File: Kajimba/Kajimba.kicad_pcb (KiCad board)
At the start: 2 copper layers, 86.4 x 49.5 mm, 17 parts, among them J1 Barrel_Jack, J2 Flow sensor JST, J3 Screen, J4 Pump GND, J5 Button, J6 Conn_01x02_Female, K1 SANYOU_SRD_Form_C, Q1 BC547, SW1 Button, U1 Pico, U2 LM7805_TO220

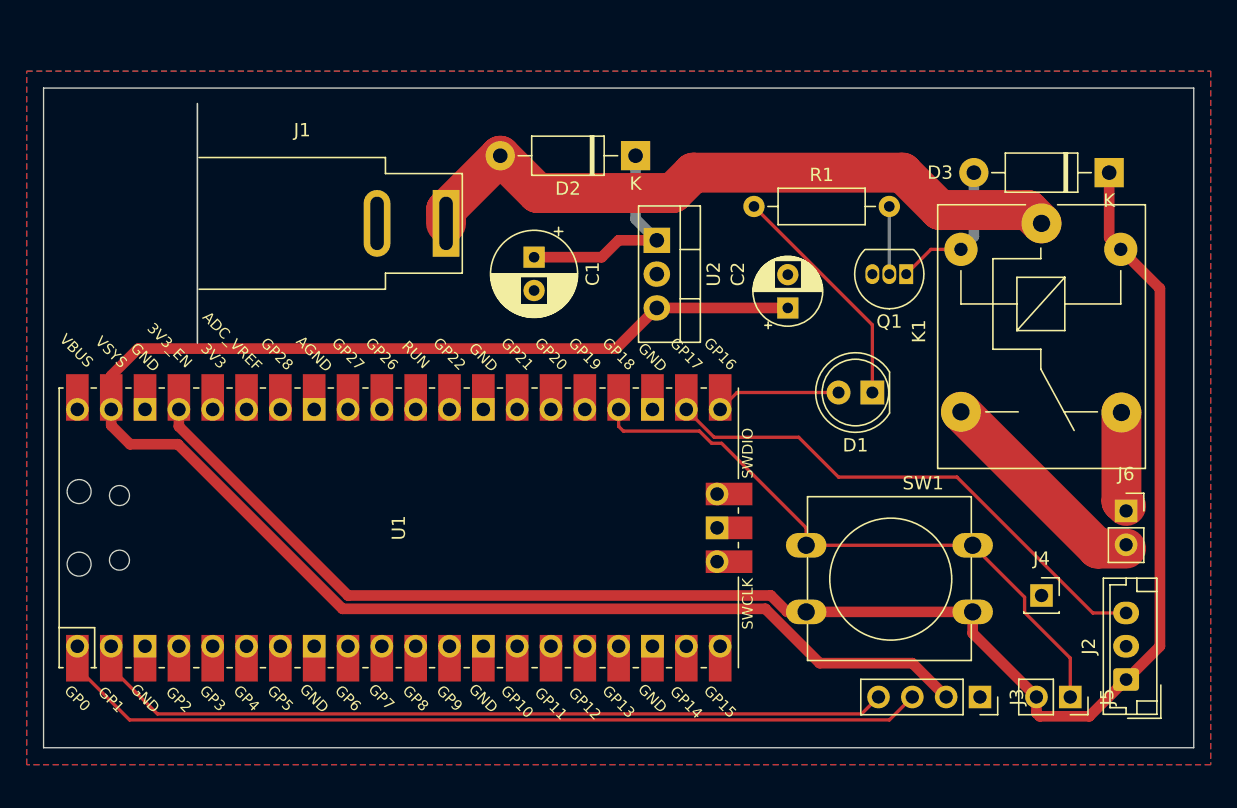
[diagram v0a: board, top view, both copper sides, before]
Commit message: KiCad PCB Pump v01.1
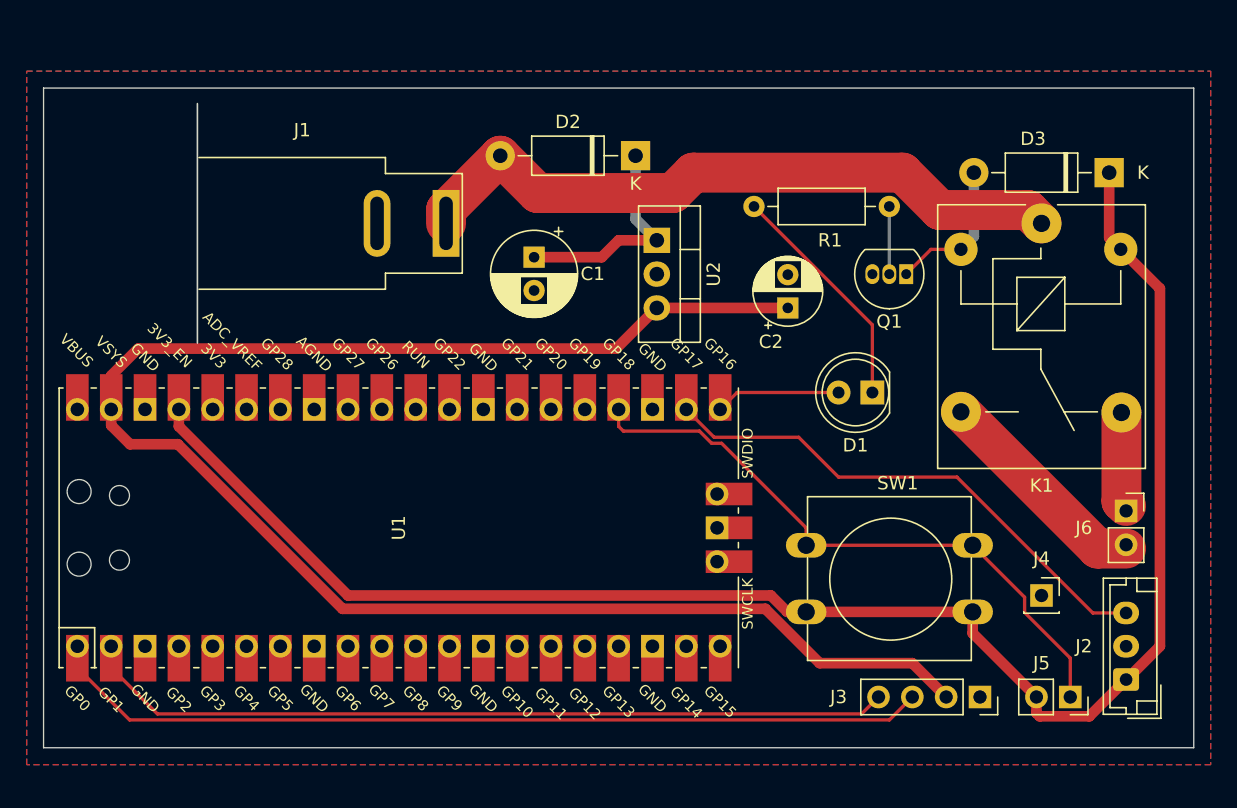
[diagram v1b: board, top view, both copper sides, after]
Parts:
- J2: value Flow sensor JST -> Flow sensor
- J6: value Conn_01x02_Female -> Relay out
- K1: value SANYOU_SRD_Form_C -> Relay
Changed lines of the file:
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@@
     (property "Sheetname" "")
     (attr through_hole)
-    (fp_text reference "D2" (at 5.08 -2.47) (layer "F.SilkS")
-      (effects (font (size 1 1) (thickness 0.15)))
-    )
-    (fp_text value "1N4007" (at 5.08 2.47) (layer "F.Fab")
+    (fp_text reference "D2" (at 5.08 2.54) (layer "F.SilkS")
+      (effects (font (size 1 1) (thickness 0.15)))
+    )
+    (fp_text value "1N4007" (at 5.08 -2.54) (layer "F.Fab")
       (effects (font (size 1 1) (thickness 0.15)))
     )
@@
     (property "Sheetname" "")
     (attr through_hole)
-    (fp_text reference "C1" (at 1.25 -4.4 90) (layer "F.SilkS")
-      (effects (font (size 1 1) (thickness 0.15)))
-    )
-    (fp_text value "470uF" (at 1.25 4.4 90) (layer "F.Fab")
+    (fp_text reference "C1" (at 1.25 -4.4 180) (layer "F.SilkS")
+      (effects (font (size 1 1) (thickness 0.15)))
+    )
+    (fp_text value "470uF" (at -3.175 0 180) (layer "F.Fab")
       (effects (font (size 1 1) (thickness 0.15)))
     )
@@
     (property "Sheetname" "")
     (attr through_hole)
-    (fp_text reference "J5" (at 0 -2.77 -90) (layer "F.SilkS")
-      (effects (font (size 1 1) (thickness 0.15)))
-    )
-    (fp_text value "Button" (at 0 5.31 -90) (layer "F.Fab")
+    (fp_text reference "J5" (at -2.54 2.159) (layer "F.SilkS")
+      (effects (font (size 1 1) (thickness 0.15)))
+    )
+    (fp_text value "Button" (at 2.54 1.524) (layer "F.Fab")
       (effects (font (size 1 1) (thickness 0.15)))
     )
@@
     (property "Sheetname" "")
     (attr through_hole)
-    (fp_text reference "J2" (at 2.5 -2.8 90) (layer "F.SilkS")
-      (effects (font (size 1 1) (thickness 0.15)))
-    )
-    (fp_text value "Flow sensor JST" (at 2.5 3.4 90) (layer "F.Fab")
+    (fp_text reference "J2" (at 2.5 -3.175 180) (layer "F.SilkS")
+      (effects (font (size 1 1) (thickness 0.15)))
+    )
+    (fp_text value "Flow sensor" (at 2.5 3.81 90) (layer "F.Fab")
       (effects (font (size 1 1) (thickness 0.15)))
     )
@@
     (property "Sheetname" "")
     (attr through_hole)
-    (fp_text reference "K1" (at 8.1 9.2 90) (layer "F.SilkS")
-      (effects (font (size 1 1) (thickness 0.15)))
-    )
-    (fp_text value "SANYOU_SRD_Form_C" (at 19.05 0 180) (layer "F.Fab")
+    (fp_text reference "K1" (at 19.685 0 180) (layer "F.SilkS")
+      (effects (font (size 1 1) (thickness 0.15)))
+    )
+    (fp_text value "Relay" (at 19.685 -1.27 180) (layer "F.Fab")
       (effects (font (size 1 1) (thickness 0.15)))
     )
@@
       (effects (font (size 1 1) (thickness 0.15)))
     )
-    (fp_text value "Barrel_Jack" (at -11 9.9) (layer "F.Fab")
+    (fp_text value "Barrel_Jack" (at -2.915 7.62) (layer "F.Fab")
       (effects (font (size 1 1) (thickness 0.15)))
     )
@@
     (property "Sheetname" "")
     (attr through_hole)
-    (fp_text reference "SW1" (at 8.78 -4.66) (layer "F.SilkS")
-      (effects (font (size 1 1) (thickness 0.15)))
-    )
-    (fp_text value "Button" (at 2.43 9.93) (layer "F.Fab")
+    (fp_text reference "SW1" (at 6.875 -4.66) (layer "F.SilkS")
+      (effects (font (size 1 1) (thickness 0.15)))
+    )
+    (fp_text value "Button" (at 2.43 -4.485) (layer "F.Fab")
       (effects (font (size 1 1) (thickness 0.15)))
     )
@@
     (property "Sheetname" "")
     (attr through_hole)
-    (fp_text reference "J3" (at 0 -2.77 -90) (layer "F.SilkS")
-      (effects (font (size 1 1) (thickness 0.15)))
-    )
-    (fp_text value "Screen" (at 0 10.39 -90) (layer "F.Fab")
+    (fp_text reference "J3" (at 0 10.62) (layer "F.SilkS")
+      (effects (font (size 1 1) (thickness 0.15)))
+    )
+    (fp_text value "Screen" (at 2.54 3.635) (layer "F.Fab")
       (effects (font (size 1 1) (thickness 0.15)))
     )
@@
     (property "Sheetname" "")
     (attr through_hole)
-    (fp_text reference "J6" (at 0 -2.77) (layer "F.SilkS")
-      (effects (font (size 1 1) (thickness 0.15)))
-    )
-    (fp_text value "Conn_01x02_Female" (at 0 5.31) (layer "F.Fab")
+    (fp_text reference "J6" (at -3.175 1.27) (layer "F.SilkS")
+      (effects (font (size 1 1) (thickness 0.15)))
+    )
+    (fp_text value "Relay out" (at 3.81 0.635 90) (layer "F.Fab")
       (effects (font (size 1 1) (thickness 0.15)))
     )
@@
     (property "Sheetname" "")
     (attr through_hole)
-    (fp_text reference "R1" (at 5.08 -2.37) (layer "F.SilkS")
-      (effects (font (size 1 1) (thickness 0.15)))
-    )
-    (fp_text value "1.5k" (at 5.08 2.37) (layer "F.Fab")
+    (fp_text reference "R1" (at 5.715 2.54) (layer "F.SilkS")
+      (effects (font (size 1 1) (thickness 0.15)))
+    )
+    (fp_text value "1.5k" (at 5.08 -2.54) (layer "F.Fab")
       (effects (font (size 1 1) (thickness 0.15)))
     )
@@
     (property "Sheetname" "")
     (attr through_hole)
-    (fp_text reference "D3" (at 12.7 0) (layer "F.SilkS")
-      (effects (font (size 1 1) (thickness 0.15)))
-    )
-    (fp_text value "1N4007" (at 5.08 2.47) (layer "F.Fab")
-      (effects (font (size 1 1) (thickness 0.15)))
-    )
-    (fp_text user "K" (at 0 -2.1) (layer "F.SilkS")
+    (fp_text reference "D3" (at 5.715 2.54) (layer "F.SilkS")
+      (effects (font (size 1 1) (thickness 0.15)))
+    )
+    (fp_text value "1N4007" (at 1.905 2.54) (layer "F.Fab")
+      (effects (font (size 1 1) (thickness 0.15)))
+    )
+    (fp_text user "K" (at -2.54 0) (layer "F.SilkS")
       (effects (font (size 1 1) (thickness 0.15)))
     )
@@
     (property "Sheetname" "")
     (attr through_hole)
-    (fp_text reference "C2" (at 2.54 -3.75 90) (layer "F.SilkS")
-      (effects (font (size 1 1) (thickness 0.15)))
-    )
-    (fp_text value "1uF" (at 1.25 3.75 90) (layer "F.Fab")
+    (fp_text reference "C2" (at -2.54 -1.27 180) (layer "F.SilkS")
+      (effects (font (size 1 1) (thickness 0.15)))
+    )
+    (fp_text value "1uF" (at -2.54 1.27 180) (layer "F.Fab")
       (effects (font (size 1 1) (thickness 0.15)))
     )
@@
     (connect_pads (clearance 0))
     (min_thickness 0.254)
-    (keepout (tracks not_allowed) (vias not_allowed) (pads not_allowed) (copperpour not_allowed) (footprints allowed))
+    (keepout (tracks not_allowed) (vias not_allowed) (pads not_allowed ) (copperpour not_allowed) (footprints allowed))
     (fill (thermal_gap 0.508) (thermal_bridge_width 0.508))
     (polygon
@@
     (connect_pads (clearance 0))
     (min_thickness 0.254)
-    (keepout (tracks not_allowed) (vias allowed) (pads allowed) (copperpour not_allowed) (footprints allowed))
+    (keepout (tracks not_allowed) (vias allowed) (pads allowed ) (copperpour not_allowed) (footprints allowed))
     (fill (thermal_gap 0.508) (thermal_bridge_width 0.508))
     (polygon
@@
     (connect_pads (clearance 0))
     (min_thickness 0.254)
-    (keepout (tracks not_allowed) (vias not_allowed) (pads not_allowed) (copperpour not_allowed) (footprints allowed))
+    (keepout (tracks not_allowed) (vias not_allowed) (pads not_allowed ) (copperpour not_allowed) (footprints allowed))
     (fill (thermal_gap 0.508) (thermal_bridge_width 0.508))
     (polygon
@@
     (connect_pads (clearance 0))
     (min_thickness 0.254)
-    (keepout (tracks not_allowed) (vias not_allowed) (pads not_allowed) (copperpour not_allowed) (footprints allowed))
+    (keepout (tracks not_allowed) (vias not_allowed) (pads not_allowed ) (copperpour not_allowed) (footprints allowed))
     (fill (thermal_gap 0.508) (thermal_bridge_width 0.508))
     (polygon

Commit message: KiCad PCB Pump v02
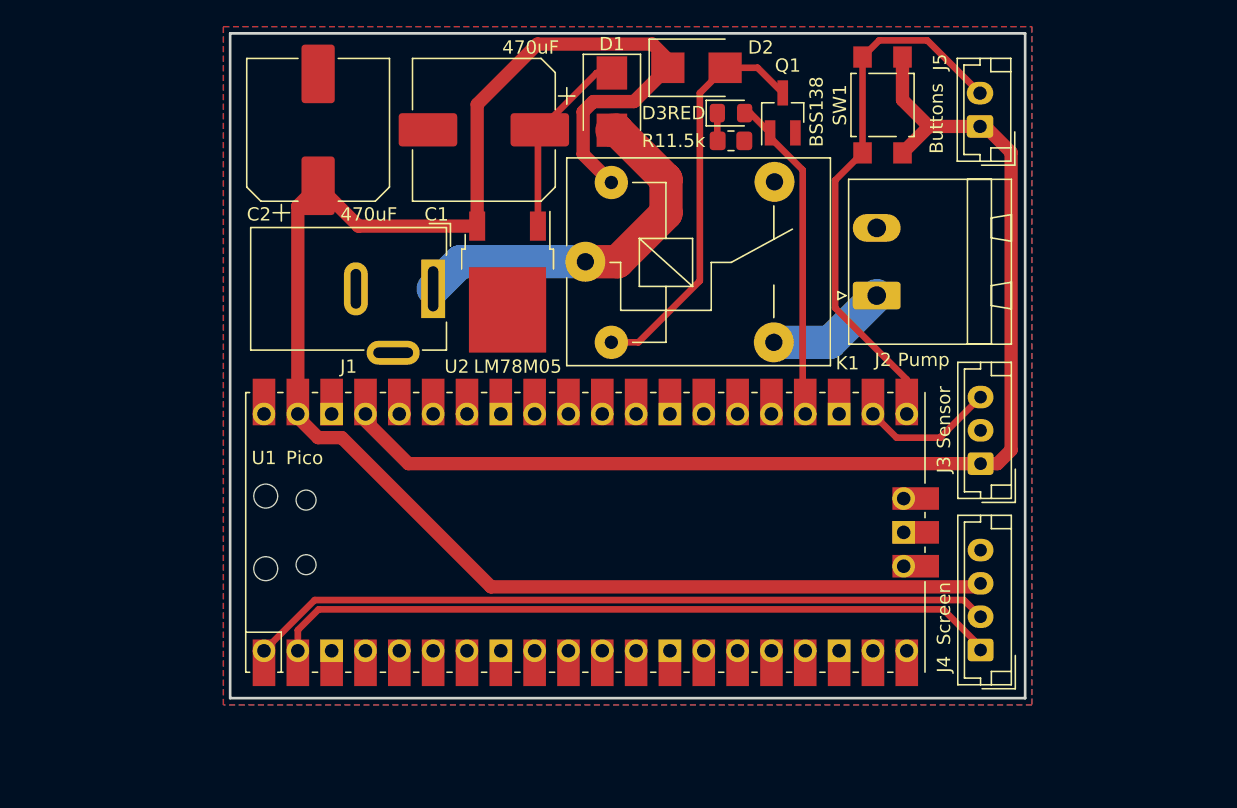
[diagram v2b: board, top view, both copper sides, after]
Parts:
- removed J6: Relay out, Connector_PinSocket_2.54mm:PinSocket_1x02_P2.54mm_Vertical
- C1: footprint Capacitor_THT:CP_Radial_D6.3mm_P2.50mm -> Capacitor_SMD:CP_Elec_10x10.5
- C2: value 1uF -> 470uF; footprint Capacitor_THT:CP_Radial_D5.0mm_P2.50mm -> Capacitor_SMD:CP_Elec_10x10.5
- D1: value RED -> S2JTR; footprint LED_THT:LED_D5.0mm -> Diode_SMD:D_SMB
- D2: value 1N4007 -> S2JTR; footprint Diode_THT:D_DO-41_SOD81_P10.16mm_Horizontal -> Diode_SMD:D_SMB
- D3: value 1N4007 -> RED; footprint Diode_THT:D_DO-41_SOD81_P10.16mm_Horizontal -> LED_SMD:LED_0805_2012Metric_Pad1.15x1.40mm_HandSolder
- J1: value Barrel_Jack -> Barrel_Jack_Switch; footprint Connector_BarrelJack:BarrelJack_SwitchcraftConxall_RAPC10U_Horizontal -> Connector_BarrelJack:BarrelJack_Wuerth_6941xx301002
- J2: value Flow sensor -> Pump; footprint Connector_JST:JST_EH_B3B-EH-A_1x03_P2.50mm_Vertical -> Connector_Phoenix_MSTB:PhoenixContact_MSTBA_2,5_2-G-5,08_1x02_P5.08mm_Horizontal
- J3: value Screen -> Sensor; footprint Connector_PinSocket_2.54mm:PinSocket_1x04_P2.54mm_Vertical -> Connector_JST:JST_EH_B3B-EH-A_1x03_P2.50mm_Vertical
- J4: value Pump GND -> Screen; footprint Connector_PinSocket_2.54mm:PinSocket_1x01_P2.54mm_Vertical -> Connector_JST:JST_EH_B4B-EH-A_1x04_P2.50mm_Vertical
- J5: footprint Connector_PinSocket_2.54mm:PinSocket_1x02_P2.54mm_Vertical -> Connector_JST:JST_EH_B2B-EH-A_1x02_P2.50mm_Vertical
- Q1: value BC547 -> BSS138; footprint Package_TO_SOT_THT:TO-92_Inline -> Package_TO_SOT_SMD:SOT-23_Handsoldering
- R1: footprint Resistor_THT:R_Axial_DIN0207_L6.3mm_D2.5mm_P10.16mm_Horizontal -> Resistor_SMD:R_0805_2012Metric_Pad1.20x1.40mm_HandSolder
- SW1: value Button -> Buttons; footprint Button_Switch_THT:SW_PUSH-12mm -> Button_Switch_SMD:SW_SPST_TL3305A
- U2: value LM7805_TO220 -> LM78M05; footprint Package_TO_SOT_THT:TO-220-3_Vertical -> Package_TO_SOT_SMD:TO-252-2
- moved J5 43.4 mm to (169.4, 75.3), turned to 90 degrees
- moved C2 37.7 mm to (119.7, 75.5)
- moved J2 34.4 mm to (161.6, 88.0)
- moved K1 34.4 mm to (139.7, 85.4), turned to 0 degrees
- moved SW1 33.6 mm to (162.1, 73.7), turned to 90 degrees
- moved D1 29.3 mm to (141.7, 73.4), turned to -90 degrees
- moved D3 28.7 mm to (150.7, 74.3), turned to 0 degrees
- moved J3 17.5 mm to (169.4, 100.6), turned to 90 degrees
- moved Q1 15.2 mm to (154.6, 74.3), turned to 90 degrees
- moved U1 14.0 mm to (139.7, 105.8)
- moved U2 11.6 mm to (133.9, 87.0)
- moved C1 10.3 mm to (132.1, 75.5), turned to 180 degrees
- moved D2 8.03 mm to (148.1, 70.9), turned to 0 degrees
- moved J4 6.14 mm to (169.4, 114.6), turned to 90 degrees
- moved R1 5.22 mm to (150.7, 76.4)
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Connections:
- D1 pad 1: Net-(D1-Pad1) -> Net-(C1-Pad1)
- D1 pad 2: Relay -> +12V
- D2 pad 1: Net-(C1-Pad1) -> +5V
- D2 pad 2: +12V -> Net-(K1-Pad2)
- D3 pad 1: +3.3V -> Net-(D3-Pad1)
- D3 pad 2: Net-(D3-Pad2) -> Relay
- J2 pad 1: +3.3V -> Net-(J2-Pad1)
- J3 pad 1: GND -> +3.3V
- J3 pad 2: +5V -> GND
- J3 pad 3: SDA -> Sensor
- J4 pad 1: GND -> SCL
- J5 pad 1: Button -> +3.3V
- J5 pad 2: +3.3V -> Button
- K1 pad 2: Net-(D3-Pad2) -> Net-(K1-Pad2)
- K1 pad 3: Net-(J6-Pad2) -> Net-(J2-Pad1)
- K1 pad 4: Net-(J6-Pad1) -> unconnected-(K1-Pad4)
- K1 pad 5: +3.3V -> +5V
- Q1 pad 1: Net-(D3-Pad2) -> Relay
- Q1 pad 2: Net-(Q1-Pad2) -> GND
- Q1 pad 3: GND -> Net-(K1-Pad2)
- R1 pad 1: Net-(D1-Pad1) -> Net-(D3-Pad1)
- R1 pad 2: Net-(Q1-Pad2) -> GND
- U1 pad 21: Relay -> Button
- U1 pad 24: Button -> Relay
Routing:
- net +3.3V: track 124.9 -> 88.9 mm
- net Net-(K1-Pad2): track 0.00 -> 30.5 mm
- net Sensor: track 39.3 -> 10.1 mm
- net +12V: track 50.8 -> 28.0 mm
- net Net-(D1-Pad1): track 17.7 -> 0.00 mm
- net Net-(J6-Pad2): track 16.7 -> 0.00 mm
- net Relay: track 9.42 -> 24.8 mm
- net Net-(D3-Pad2): track 11.0 -> 0.00 mm
- net SDA: track 66.6 -> 55.9 mm
- net Net-(J2-Pad1): track 0.00 -> 9.18 mm
- net Net-(J6-Pad1): track 7.16 -> 0.00 mm
- net SCL: track 61.2 -> 54.9 mm
- net Button: track 46.7 -> 40.9 mm
- net Net-(Q1-Pad2): track 5.08 -> 0.00 mm
- net Net-(C1-Pad1): track 16.8 -> 14.5 mm
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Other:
- board size 86.4 x 49.5 mm -> 59.7 x 49.9 mm
- board text added: "+"
- board text added: "-"
- board text added: "v02 Kajimba Pump"
- board text removed: "v01"

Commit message: KiCad PCB Pump v03
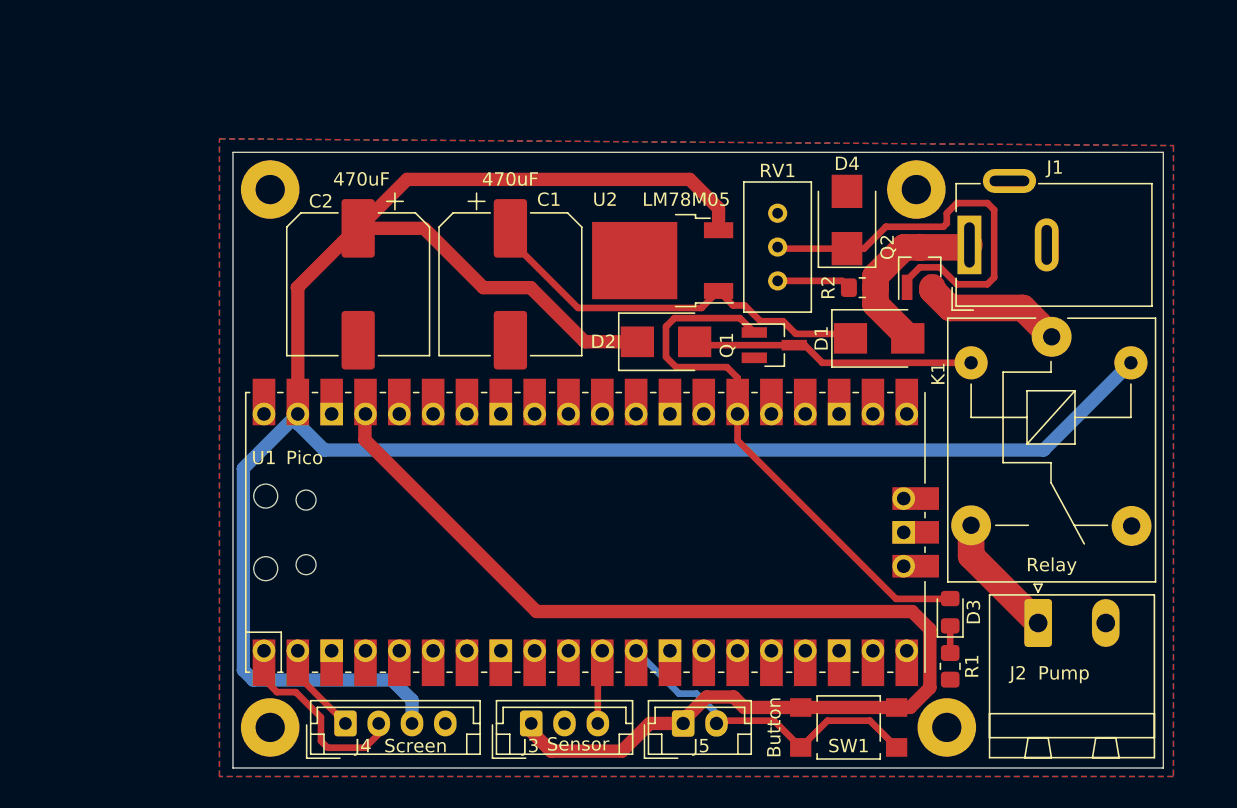
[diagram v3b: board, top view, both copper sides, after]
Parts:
- added D4: S2JTR, Diode_SMD:D_SMB, F.Cu at (159.4, 82.3)
- added H1: GND_Pad, MountingHole:MountingHole_2.2mm_M2_Pad, F.Cu at (116.1, 120.4)
- added H2: GND_Pad, MountingHole:MountingHole_2.2mm_M2_Pad, F.Cu at (164.6, 80.0)
- added H3: GND_Pad, MountingHole:MountingHole_2.2mm_M2_Pad, F.Cu at (166.9, 120.4)
- added H4: GND_Pad, MountingHole:MountingHole_2.2mm_M2_Pad, F.Cu at (116.1, 80.0)
- added Q2: BSS138, Package_TO_SOT_SMD:SOT-23_Handsoldering, F.Cu at (164.8, 85.9)
- added R2: 470, Resistor_SMD:R_0805_2012Metric_Pad1.20x1.40mm_HandSolder, F.Cu at (160.5, 87.4)
- added RV1: R_Potentiometer, Potentiometer_THT:Potentiometer_Bourns_3296W_Vertical, F.Cu at (154.2, 86.9)
- SW1: value Buttons -> Button
- moved J5 50.1 mm to (147.1, 120.1), turned to 0 degrees
- moved J4 48.0 mm to (121.7, 120.1), turned to 0 degrees
- moved SW1 46.8 mm to (159.5, 120.4), turned to 180 degrees
- moved R1 42.8 mm to (167.1, 115.8), turned to -90 degrees
- moved D3 40.9 mm to (167.1, 111.7), turned to 90 degrees
- moved J1 40.4 mm to (168.6, 84.2), turned to 90 degrees
- moved J3 39.0 mm to (135.7, 120.1), turned to 0 degrees
- moved K1 35.5 mm to (174.8, 91.1), turned to -90 degrees
- moved J2 27.4 mm to (173.7, 112.6), turned to 0 degrees
- moved D1 26.8 mm to (161.8, 91.2), turned to 0 degrees
- moved D2 20.7 mm to (145.8, 91.4)
- moved Q1 17.5 mm to (153.9, 91.7), turned to 0 degrees
- moved C2 12.0 mm to (122.7, 87.1), turned to -90 degrees
- moved C1 11.8 mm to (134.1, 87.1), turned to -90 degrees
- moved U2 11.8 mm to (145.5, 85.3), turned to 180 degrees
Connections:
- K1 pad 1: +12V -> Pump
- U1 pad 11: unconnected-(U1-Pad11) -> Sensor
- U1 pad 12: unconnected-(U1-Pad12) -> Button
- U1 pad 21: Button -> unconnected-(U1-Pad21)
- U1 pad 22: Sensor -> unconnected-(U1-Pad22)
- U1 pad 24: Relay -> unconnected-(U1-Pad24)
- U1 pad 26: unconnected-(U1-Pad26) -> Relay
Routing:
- net SCL: track 54.9 -> 6.94 mm
- net +5V: track 128.2 -> 174.6 mm
- net SDA: track 55.9 -> 15.1 mm
- net Net-(D4-Pad1): track 0.00 -> 31.7 mm
- net Relay: track 24.8 -> 41.2 mm
- net Net-(C1-Pad1): track 14.5 -> 30.5 mm
- net Button: track 40.9 -> 25.2 mm
- net +12V: track 28.0 -> 13.7 mm
- net Pump: track 0.00 -> 10.6 mm
- net Net-(D2-Pad2): track 30.5 -> 20.6 mm
- net Net-(R2-Pad1): track 0.00 -> 5.56 mm
- net Sensor: track 10.1 -> 5.59 mm
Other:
- board size 59.7 x 49.9 mm -> 69.8 x 46.2 mm
- board text added: "v03 Kajimba Pump"
- board text removed: "v02 Kajimba Pump"
